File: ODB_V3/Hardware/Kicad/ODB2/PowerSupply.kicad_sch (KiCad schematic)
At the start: 53 parts, among them U13 L6981N33DR, U7 MPQ9843GLE-5-AEC1-Z

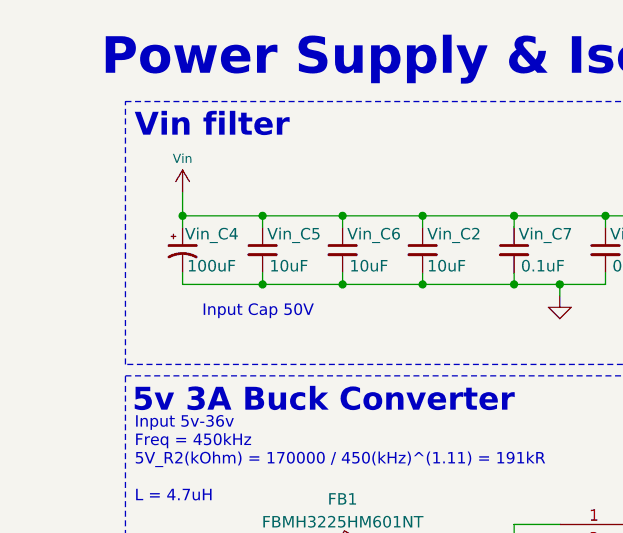
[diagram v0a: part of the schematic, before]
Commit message: chore: update some footprint
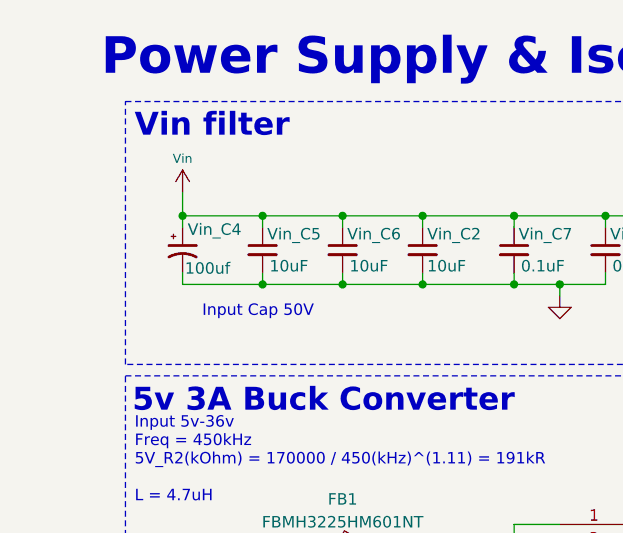
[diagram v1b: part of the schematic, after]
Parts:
- removed Vin_C4: 100uF, symbol Device:C_Polarized_Small_US
- added Vin_C4: 100uf, ODB:WCAP-PSHP_8X8.7_DXL_, symbol ODB2:875115652007
- NT1, NT2, NT3, NT4: footprint (none) -> NetTie:NetTie-2_SMD_Pad0.5mm
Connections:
- net GND: now also Vin_C4.2
- net Vin: now also Vin_C4.1
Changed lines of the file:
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@@
 			)
 		)
-		(property "Footprint" ""
+		(property "Footprint" "NetTie:NetTie-2_SMD_Pad0.5mm"
 			(at 110.49 181.61 0)
 			(effects
@@
 	)
 	(symbol
-		(lib_id "Device:C_Polarized_Small_US")
-		(at 21.59 38.1 0)
-		(unit 1)
-		(exclude_from_sim no)
-		(in_bom yes)
-		(on_board yes)
-		(dnp no)
-		(property "Reference" "Vin_C4"
-			(at 21.844 36.322 0)
-			(effects
-				(font
-					(size 1.27 1.27)
-				)
-				(justify left)
-			)
-		)
-		(property "Value" "100uF"
-			(at 22.098 39.878 0)
-			(effects
-				(font
-					(size 1.27 1.27)
-				)
-				(justify left)
-			)
-		)
-		(property "Footprint" ""
-			(at 21.59 38.1 0)
-			(effects
-				(font
-					(size 1.27 1.27)
-				)
-				(hide yes)
-			)
-		)
-		(property "Datasheet" "~"
-			(at 21.59 38.1 0)
-			(effects
-				(font
-					(size 1.27 1.27)
-				)
-				(hide yes)
-			)
-		)
-		(property "Description" "Polarized capacitor, small US symbol"
-			(at 21.59 38.1 0)
-			(effects
-				(font
-					(size 1.27 1.27)
-				)
-				(hide yes)
-			)
-		)
-		(pin "1"
-		)
-		(pin "2"
-		)
-		(instances
-			(project ""
-				(path "/4b06c5d1-aa8b-48ed-8972-b43a60cfab78/a0dfa29e-ccca-4096-8481-c7e33c67aac5"
-					(reference "Vin_C4")
-					(unit 1)
-				)
-			)
-		)
-	)
-	(symbol
 		(lib_id "power:GND")
 		(at 265.43 33.02 0)
@@
 	)
 	(symbol
+		(lib_id "ODB2:875115652007")
+		(at 21.59 38.1 0)
+		(unit 1)
+		(exclude_from_sim no)
+		(in_bom yes)
+		(on_board yes)
+		(dnp no)
+		(property "Reference" "Vin_C4"
+			(at 25.146 35.814 0)
+			(effects
+				(font
+					(size 1.27 1.27)
+				)
+			)
+		)
+		(property "Value" "100uf"
+			(at 21.844 40.132 0)
+			(effects
+				(font
+					(size 1.27 1.27)
+				)
+				(justify left)
+			)
+		)
+		(property "Footprint" "ODB:WCAP-PSHP_8X8.7_DXL_"
+			(at 21.59 38.1 0)
+			(effects
+				(font
+					(size 1.27 1.27)
+				)
+				(hide yes)
+			)
+		)
+		(property "Datasheet" "https://www.digikey.ca/en/products/detail/w%C3%BCrth-elektronik/875115652007/8556615"
+			(at 21.59 38.1 0)
+			(effects
+				(font
+					(size 1.27 1.27)
+				)
+				(hide yes)
+			)
+		)
+		(property "Description" "CAP ALUM POLY 100UF 20% 35V SMD"
+			(at 21.59 38.1 0)
+			(effects
+				(font
+					(size 1.27 1.27)
+				)
+				(hide yes)
+			)
+		)
+		(pin "1"
+		)
+		(pin "2"
+		)
+		(instances
+			(project ""
+				(path "/4b06c5d1-aa8b-48ed-8972-b43a60cfab78/a0dfa29e-ccca-4096-8481-c7e33c67aac5"
+					(reference "Vin_C4")
+					(unit 1)
+				)
+			)
+		)
+	)
+	(symbol
 		(lib_id "power:GND")
 		(at 50.8 80.01 0)
@@
 			)
 		)
-		(property "Footprint" ""
+		(property "Footprint" "NetTie:NetTie-2_SMD_Pad0.5mm"
 			(at 110.49 186.69 0)
 			(effects
@@
 			)
 		)
-		(property "Footprint" ""
+		(property "Footprint" "NetTie:NetTie-2_SMD_Pad0.5mm"
 			(at 144.78 101.6 0)
 			(effects
@@
 			)
 		)
-		(property "Footprint" ""
+		(property "Footprint" "NetTie:NetTie-2_SMD_Pad0.5mm"
 			(at 144.78 107.95 0)
 			(effects
